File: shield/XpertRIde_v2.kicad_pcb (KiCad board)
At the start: 2 copper layers, 55.3 x 50.5 mm, 44 parts, among them J1 Conn_01x20, J2 USB_B_Micro, J3 Conn_02x05_Counter_Clockwise, J4 Conn_01x01_Female, J5 Conn_01x01_Female, J6 Conn_01x01_Female, J7 Conn_01x05, SW1 SW_DPDT_x2, U1 MCP6N11-001, U2 ADG728, U3 ADG728, U4 ADG728, U5 AD5245-100k

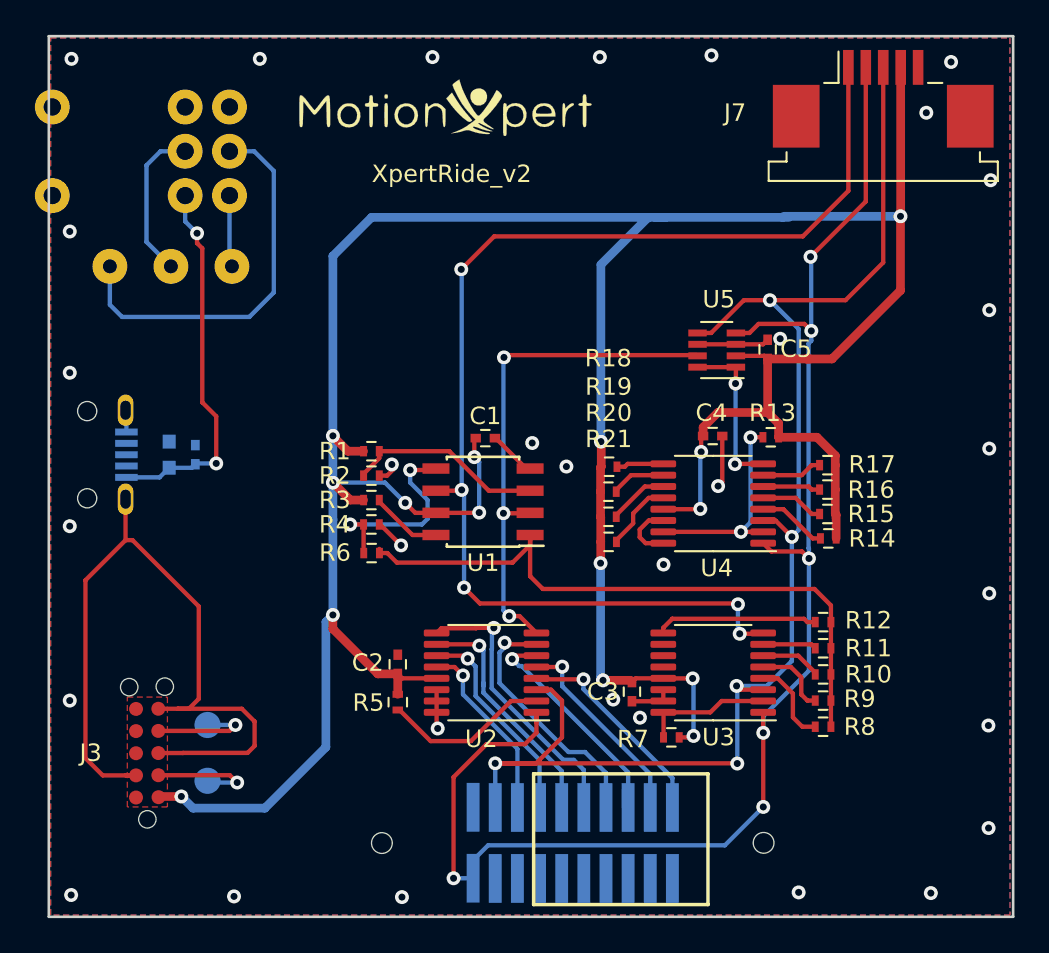
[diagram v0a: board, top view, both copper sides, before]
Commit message: new design
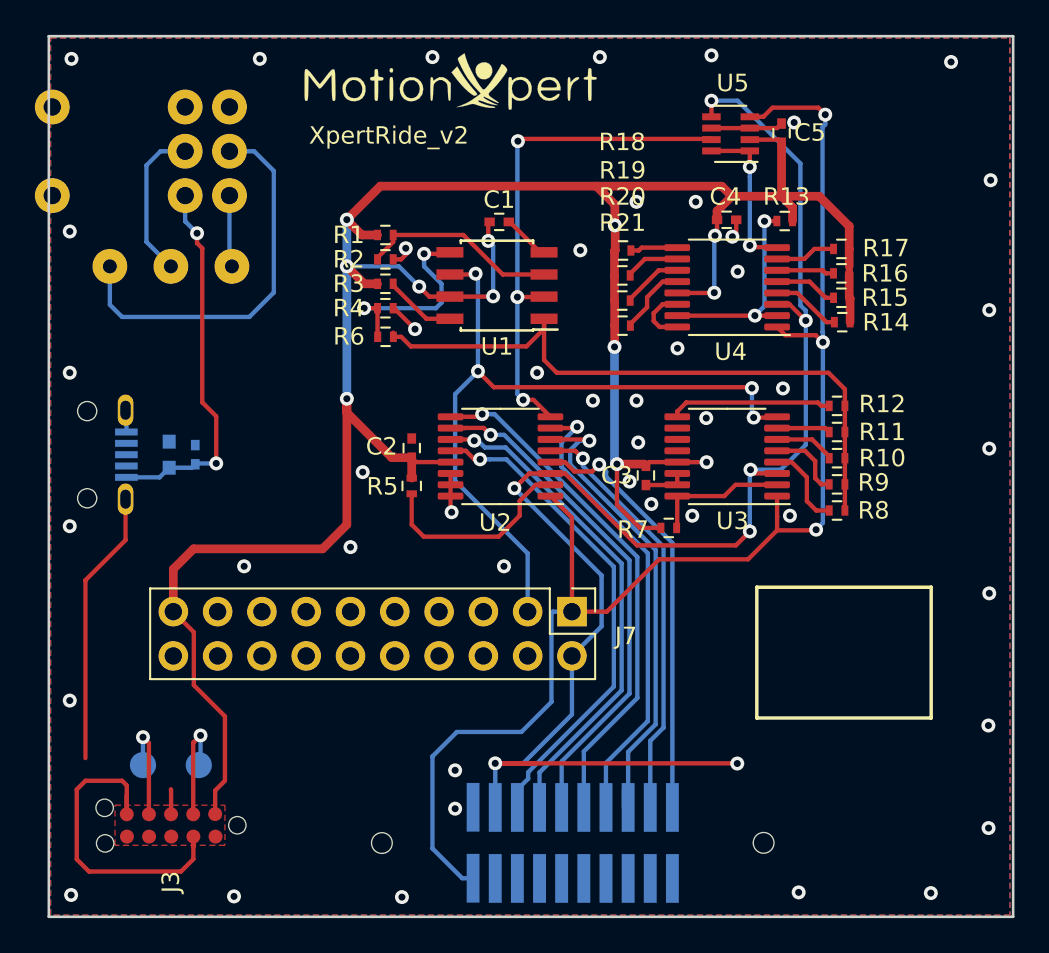
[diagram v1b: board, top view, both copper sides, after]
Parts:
- J7: value Conn_01x05 -> Conn_02x10_Odd_Even; footprint Connector_FFC-FPC:TE_84952-5_1x05-1MP_P1.0mm_Horizontal -> Pin_Headers:Pin_Header_Straight_2x10_Pitch2.54mm
- moved J7 34.4 mm to (68.9, 103.0), turned to 270 degrees
- moved R18 12.4 mm to (71.9, 82.3)
- moved U5 12.4 mm to (78.0, 75.6)
- moved C1 12.4 mm to (64.8, 80.7)
- moved C2 12.4 mm to (59.8, 93.7)
- moved C4 12.4 mm to (77.8, 80.6)
- moved C5 12.4 mm to (81.0, 75.6)
- moved R1 12.4 mm to (58.2, 81.4)
- moved R10 12.4 mm to (84.1, 94.2)
- moved R11 12.4 mm to (84.1, 92.7)
- moved R12 12.4 mm to (84.1, 91.2)
- moved R13 12.4 mm to (81.1, 80.6)
- moved R14 12.4 mm to (84.4, 86.4)
- moved R16 12.4 mm to (84.4, 83.6)
- moved R17 12.4 mm to (84.4, 82.2)
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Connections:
- J7 pad 1: /AMP_OUT -> /TWI_CLK
- J7 pad 2: /TWI_CLK -> /TWI_SDA
- J7 pad 3: /TWI_SDA -> /AMP_OUT
- J7 pad 4: VDD -> (no net)
- J7 pad 5: GNDD -> (no net)
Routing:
- net VDD: track 186.7 -> 149.1 mm, vias 15 -> 12
- net /AMP_OUT: track 70.2 -> 42.4 mm, vias 5 -> 4
- net /Sensor8: track 10.6 -> 28.2 mm
- net /Sensor7: track 12.1 -> 28.7 mm
- net /Sensor6: track 13.9 -> 29.2 mm
- net /Sensor3: track 13.9 -> 27.8 mm
- net /Sensor5: track 16.3 -> 29.8 mm
- net /Sensor2: track 12.7 -> 25.3 mm
- net /Sensor1: track 13.2 -> 25.7 mm
- net /Sensor4: track 14.5 -> 26.8 mm
- net GNDD: track 67.4 -> 56.7 mm, vias 32 -> 47
- net /TWI_SDA: track 81.6 -> 90.8 mm, vias 5 -> 7
- net /TWI_CLK: track 86.9 -> 80.6 mm, vias 6 -> 3
- net Net-(R5-Pad1): track 9.64 -> 11.8 mm
